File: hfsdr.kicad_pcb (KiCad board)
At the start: 2 copper layers, 91 parts, among them J1 RFIN, U2 ADA4938-1, U4 AD9515

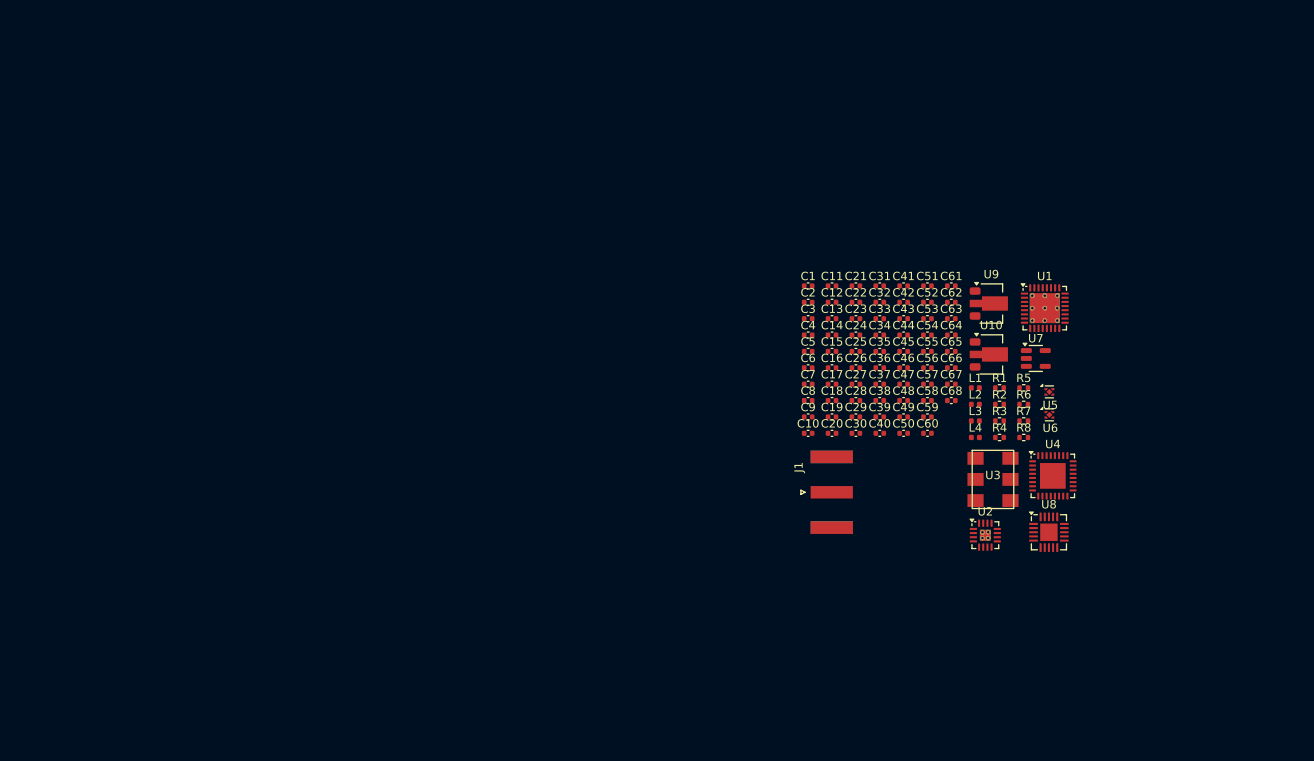
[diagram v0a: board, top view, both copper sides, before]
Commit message: dgfsd
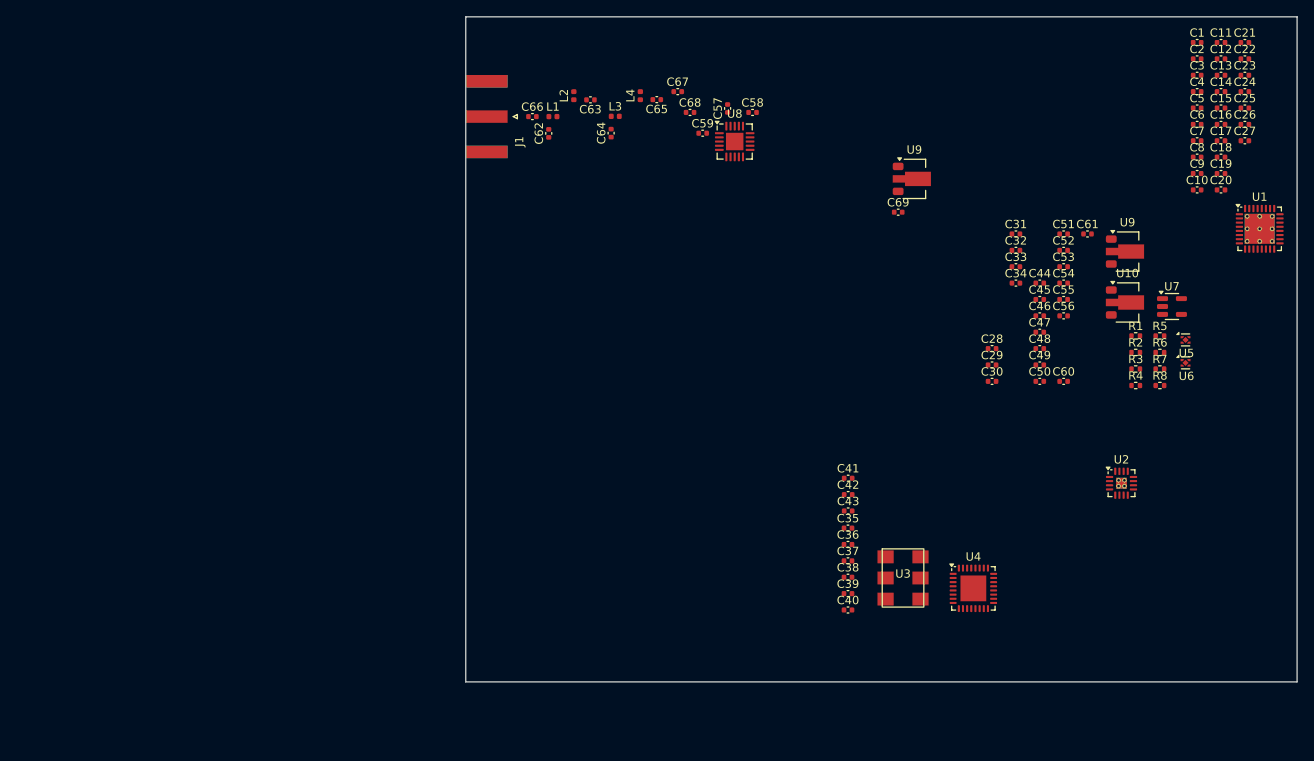
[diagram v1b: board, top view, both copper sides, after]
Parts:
- added C69: 0.1uF, Capacitor_SMD:C_0402_1005Metric, F.Cu at (167.0, 93.5)
- added U9: AP2205-50Y-13, Package_TO_SOT_SMD:SOT-89-3, F.Cu at (169.0, 89.5)
- U10: value ~ -> AP2205-50Y-13
- U7: value ~ -> TLV77333PDBVR
- U8: value ~ -> ADL5206
- moved J1 61.4 mm to (117.5, 82.0), turned to 180 degrees
- moved L2 60.9 mm to (128.0, 79.5), turned to 90 degrees
- moved L1 60.4 mm to (125.5, 82.0)
- moved U8 60.3 mm to (147.3, 85.0)
- moved C66 58.8 mm to (123.0, 82.0)
- moved L4 57.6 mm to (136.0, 79.5), turned to 90 degrees
- moved L3 56.7 mm to (133.0, 82.0)
- moved C1 55.2 mm to (203.0, 73.1)
- moved C10 55.2 mm to (203.0, 90.8)
- moved C11 55.2 mm to (205.8, 73.1)
- moved C12 55.2 mm to (205.8, 75.1)
- moved C13 55.2 mm to (205.8, 77.0)
- moved C14 55.2 mm to (205.8, 79.0)
- moved C15 55.2 mm to (205.8, 81.0)
- moved C16 55.2 mm to (205.8, 82.9)
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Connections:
- C19 pad 2: AGND -> DRGND
- C20 pad 2: AGND -> DRGND
- C21 pad 2: AGND -> DRGND
- C22 pad 2: AGND -> DRGND
- C23 pad 2: AGND -> DRGND
- C24 pad 2: AGND -> DRGND
- C25 pad 2: AGND -> DRGND
- C26 pad 2: AGND -> DRGND
- U2 pad 14: -5V -> -5V_1
- U2 pad 15: -5V -> -5V_3
- U2 pad 16: -5V -> -5V_2
- U8 pad 6: VGA_CSB -> unconnected-(U8-CS/GS1/D3-Pad6)
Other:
- board outline added: 100 x 80 mm
- copper layers 2 -> 4

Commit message: some more fpga work
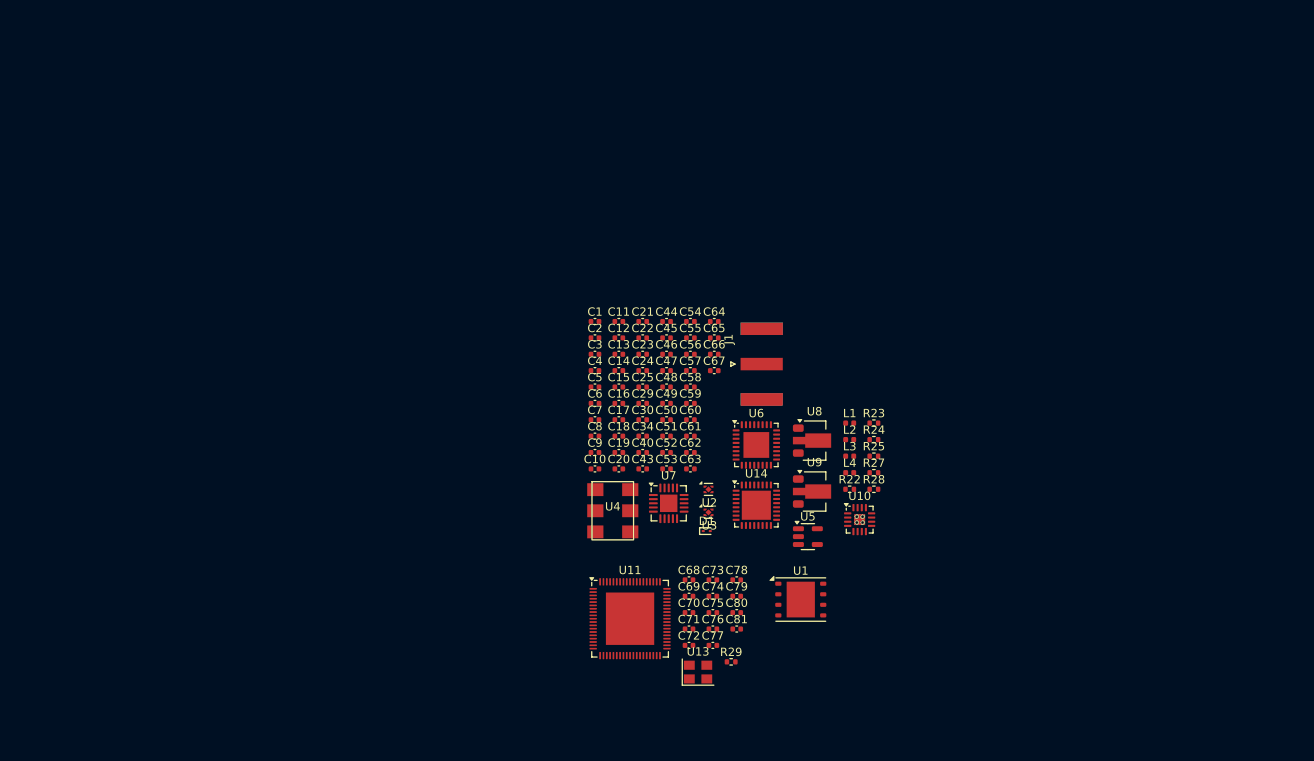
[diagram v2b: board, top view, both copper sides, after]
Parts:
- removed C26: 1uF, Capacitor_SMD:C_0402_1005Metric
- removed C27, C33, C35, C36, C37, C38, C39, C41, C42: 0.1uF, Capacitor_SMD:C_0402_1005Metric
- removed C28: 15pF, Capacitor_SMD:C_0402_1005Metric
- removed C31, C32: 0.1u, Capacitor_SMD:C_0402_1005Metric
- removed R1, R2: 250, Resistor_SMD:R_0402_1005Metric
- removed R3, R5: 33, Resistor_SMD:R_0402_1005Metric
- removed R4, R6: 15, Resistor_SMD:R_0402_1005Metric
- removed R7, R8: 50, Resistor_SMD:R_0402_1005Metric
- removed the U9 at (194.6, 98.2)
- removed the U9 at (169.0, 89.5)
- added C70: 100n, Capacitor_SMD:C_0402_1005Metric, F.Cu at (141.9, 141.7)
- added C71: 100n, Capacitor_SMD:C_0402_1005Metric, F.Cu at (141.9, 143.6)
- added C72: 100n, Capacitor_SMD:C_0402_1005Metric, F.Cu at (141.9, 145.6)
- added C73: 100u, Capacitor_SMD:C_0402_1005Metric, F.Cu at (144.7, 137.7)
- added C74: 4.7u, Capacitor_SMD:C_0402_1005Metric, F.Cu at (144.7, 139.7)
- added C75: 0.1u, Capacitor_SMD:C_0402_1005Metric, F.Cu at (144.7, 141.7)
- added C76: 0.1u, Capacitor_SMD:C_0402_1005Metric, F.Cu at (144.7, 143.6)
- added C77: 26p, Capacitor_SMD:C_0402_1005Metric, F.Cu at (144.7, 145.6)
- added C78: 26p, Capacitor_SMD:C_0402_1005Metric, F.Cu at (147.6, 137.7)
- added C79: 0.1uF, Capacitor_SMD:C_0402_1005Metric, F.Cu at (147.6, 139.7)
- added C80: 0.1uF, Capacitor_SMD:C_0402_1005Metric, F.Cu at (147.6, 141.7)
- added C81: 0.1uF, Capacitor_SMD:C_0402_1005Metric, F.Cu at (147.6, 143.6)
- added D1: ESD9B3.3ST5G, Diode_SMD:D_SOD-923, F.Cu at (144.0, 131.9)
- added R22: 50, Resistor_SMD:R_0402_1005Metric, F.Cu at (161.2, 126.8)
- added R23: 50, Resistor_SMD:R_0402_1005Metric, F.Cu at (164.1, 118.9)
- added R24: 250, Resistor_SMD:R_0402_1005Metric, F.Cu at (164.1, 120.9)
- added R25: 250, Resistor_SMD:R_0402_1005Metric, F.Cu at (164.1, 122.8)
- added R27: 33, Resistor_SMD:R_0402_1005Metric, F.Cu at (164.1, 124.8)
- added R28: 33, Resistor_SMD:R_0402_1005Metric, F.Cu at (164.1, 126.8)
- added R29: 1.6K 1%, Resistor_SMD:R_0402_1005Metric, F.Cu at (146.9, 147.6)
- added U11: FT601Q, Package_DFN_QFN:QFN-76-1EP_9x9mm_P0.4mm_EP5.81x6.31mm, F.Cu at (134.8, 142.4)
- added U13: ABM8-30.000MHZ-D1X-T, Oscillator:Oscillator_SMD_Abracon_ASE-4Pin_3.2x2.5mm, F.Cu at (142.9, 148.8)
- added U14: AD9649, Package_CSP:LFCSP-32-1EP_5x5mm_P0.5mm_EP3.5x3.5mm, F.Cu at (150.0, 128.8)
- added U9: AP2205-50Y-13, Package_TO_SOT_SMD:SOT-89-3, F.Cu at (157.0, 127.1)
- C10, C13, C15, C16, C17, C18, C24, C25, C34, C44, C45, C46, C49: value 1uF -> 0.1uF
- C19, C2, C5, C59, C6, C8, C9: value 0.1uF -> 1uF
- C29: value 5pF -> 1uF
- C30: value 15pF -> 0.1uF
- C47: value 1uF -> 0.1u
- C48: value 0.1uF -> 0.1u
- C51: value 0.1n -> 1uF
- C53: value 0.1uF -> 0.1n
- C57: value 0.1uF -> 470n
- C58: value 0.1uF -> 120p
- C60: value 1uF -> 200p
- C61: value 2.2uF -> 200p
- C62: value 120p -> 2.2uF
- C63: value 200p -> 160p
- C64: value 200p -> 0.1u
- C65: value 160p -> 0.1u
- C66: value 470n -> 0.1uF
- C67: value 0.1u -> 22pF
- C68: value 0.1u -> 100n
- C69: value 0.1uF -> 100n
- U1: value ~ -> W25Q128JVP; footprint Package_CSP:LFCSP-32-1EP_5x5mm_P0.5mm_EP3.6x3.6mm_ThermalVias -> Package_SON:WSON-8-1EP_6x5mm_P1.27mm_EP3.4x4.3mm
- U10: value AP2205-50Y-13 -> ADA4938-1; footprint Package_TO_SOT_SMD:SOT-89-3 -> Package_CSP:LFCSP-16-1EP_3x3mm_P0.5mm_EP1.3x1.3mm_ThermalVias
- U2: value ADA4938-1 -> ~; footprint Package_CSP:LFCSP-16-1EP_3x3mm_P0.5mm_EP1.3x1.3mm_ThermalVias -> Package_DFN_QFN:OnSemi_XDFN4-1EP_1.0x1.0mm_EP0.52x0.52mm
- U3: footprint hfsdr:SI590_5x7mm -> Package_DFN_QFN:OnSemi_XDFN4-1EP_1.0x1.0mm_EP0.52x0.52mm
- U4: value AD9515 -> ~; footprint Package_CSP:LFCSP-32-1EP_5x5mm_P0.5mm_EP3.1x3.1mm -> hfsdr:SI590_5x7mm
- U5: value ~ -> TLV77333PDBVR; footprint Package_DFN_QFN:OnSemi_XDFN4-1EP_1.0x1.0mm_EP0.52x0.52mm -> Package_TO_SOT_SMD:SOT-23-5
- U6: value ~ -> AD9515; footprint Package_DFN_QFN:OnSemi_XDFN4-1EP_1.0x1.0mm_EP0.52x0.52mm -> Package_CSP:LFCSP-32-1EP_5x5mm_P0.5mm_EP3.1x3.1mm
- U7: value TLV77333PDBVR -> ADL5206; footprint Package_TO_SOT_SMD:SOT-23-5 -> Package_CSP:LFCSP-20-1EP_4x4mm_P0.5mm_EP2.1x2.1mm
- U8: value ADL5206 -> AP2205-50Y-13; footprint Package_CSP:LFCSP-20-1EP_4x4mm_P0.5mm_EP2.1x2.1mm -> Package_TO_SOT_SMD:SOT-89-3
- moved C1 79.8 mm to (130.5, 106.7)
- moved C10 79.8 mm to (130.5, 124.4)
- moved C11 79.8 mm to (133.4, 106.7)
- moved C12 79.8 mm to (133.4, 108.6)
- moved C13 79.8 mm to (133.4, 110.6)
- moved C14 79.8 mm to (133.4, 112.6)
- moved C15 79.8 mm to (133.4, 114.5)
- moved C16 79.8 mm to (133.4, 116.5)
- moved C17 79.8 mm to (133.4, 118.5)
- moved C18 79.8 mm to (133.4, 120.4)
- moved C19 79.8 mm to (133.4, 122.4)
- moved C2 79.8 mm to (130.5, 108.6)
- moved C20 79.8 mm to (133.4, 124.4)
- moved C21 79.8 mm to (136.3, 106.7)
- moved C22 79.8 mm to (136.3, 108.6)
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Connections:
- C10 pad 1: AVDD -> CLKVDD
- C12 pad 1: AVDD -> DRVDD
- C15 pad 1: AVDD -> VCM
- C16 pad 1: AVDD -> CLKVDD
- C18 pad 1: AVDD -> VREF
- C19 pad 1: DRVDD -> VREF
- C19 pad 2: DRGND -> AGND
- C20 pad 1: DRVDD -> CLKVDD
- C20 pad 2: DRGND -> AGND
- C21 pad 1: DRVDD -> Net-(C21-Pad1)
- C21 pad 2: DRGND -> CLK-
- C22 pad 1: DRVDD -> Net-(C22-Pad1)
- C22 pad 2: DRGND -> CLK+
- C23 pad 2: DRGND -> AGND
- C24 pad 1: DRVDD -> CLKVDD
- C24 pad 2: DRGND -> AGND
- C25 pad 1: DRVDD -> CLKVDD
- C25 pad 2: DRGND -> AGND
- C29 pad 1: Net-(C29-Pad1) -> CLKVDD
- C29 pad 2: Net-(C28-Pad1) -> AGND
- C3 pad 1: AVDD -> DRVDD
- C30 pad 1: AGND -> CLKVDD
- C30 pad 2: Net-(C29-Pad1) -> AGND
- C4 pad 1: AVDD -> CLKVDD
- C44 pad 1: +5V -> VCM
- C45 pad 1: AVDD -> VGA_VDD
- C46 pad 1: +5V -> AGND
- C46 pad 2: AGND -> Net-(U6-S6)
- C47 pad 1: DRVDD -> Net-(U4-CLK+)
- C47 pad 2: AGND -> Net-(U6-CLK)
- C48 pad 1: AGND -> Net-(U4-CLK-)
- C48 pad 2: Net-(U4-S6) -> Net-(U6-CLKB)
- C49 pad 1: +5V -> VGA_VDD
- C5 pad 1: AVDD -> +5V
- C50 pad 1: CLKVDD -> +5V
- C51 pad 1: Net-(U4-OUT0B) -> CLKVDD
- C51 pad 2: CLK- -> AGND
- C52 pad 1: Net-(U4-OUT0) -> Net-(U6-OUT0B)
- C52 pad 2: CLK+ -> Net-(C21-Pad1)
- C53 pad 1: Net-(U1-CLK-) -> Net-(U6-OUT0)
- C53 pad 2: CLK- -> Net-(C22-Pad1)
- C54 pad 1: Net-(U1-CLK+) -> AGND
- C54 pad 2: CLK+ -> Net-(U7-VCM)
- C57 pad 1: VGA_VDD -> Net-(D1-A2)
- C57 pad 2: AGND -> Net-(C57-Pad2)
- C58 pad 1: VGA_VDD -> Net-(C57-Pad2)
- C59 pad 1: AGND -> +13.8V
- C59 pad 2: Net-(U8-VCM) -> AGND
- C6 pad 1: AVDD -> +5V
- C60 pad 1: +13.8V -> Net-(C60-Pad1)
- C61 pad 1: Net-(U10-VOUT) -> Net-(C61-Pad1)
- C62 pad 1: Net-(C62-Pad1) -> Net-(U9-VOUT)
- C64 pad 2: AGND -> AMPIN+
- C65 pad 1: Net-(C65-Pad1) -> AGND
- C65 pad 2: AGND -> AMPIN-
- C66 pad 1: Net-(J1-In) -> AGND
- C66 pad 2: Net-(C62-Pad1) -> Net-(U9-VOUT)
- C67 pad 1: Net-(C67-Pad1) -> ADCIN-
- C67 pad 2: AMPIN+ -> ADCIN+
- C68 pad 1: AGND -> Net-(J2-TX1-)
- C68 pad 2: AMPIN- -> Net-(U12-TX1n)
- C69 pad 1: AGND -> Net-(J2-TX1+)
- C69 pad 2: Net-(U10-VOUT) -> Net-(U12-TX1p)
- J1 pad 1: Net-(J1-In) -> Net-(D1-A2)
- L1 pad 1: Net-(C62-Pad1) -> Net-(C57-Pad2)
- L1 pad 2: Net-(C63-Pad1) -> Net-(C60-Pad1)
- L2 pad 1: Net-(C63-Pad1) -> Net-(C60-Pad1)
- L2 pad 2: Net-(C64-Pad1) -> Net-(C61-Pad1)
- L3 pad 1: Net-(C64-Pad1) -> Net-(C61-Pad1)
- L3 pad 2: Net-(C65-Pad1) -> Net-(C63-Pad1)
- L4 pad 1: Net-(C65-Pad1) -> Net-(C63-Pad1)
- L4 pad 2: Net-(C67-Pad1) -> Net-(C64-Pad1)
- U1 pad 1: AVDD -> unconnected-(U1-~{CS}-Pad1)
- U1 pad 3: AVDD -> unconnected-(U1-IO2-Pad3)
- U1 pad 4: Net-(U1-CLK+) -> unconnected-(U1-GND-Pad4)
- U1 pad 5: Net-(U1-CLK-) -> unconnected-(U1-DI(IO0)-Pad5)
- U1 pad 6: AVDD -> unconnected-(U1-CLK-Pad6)
- U1 pad 8: AVDD -> unconnected-(U1-VCC-Pad8)
- U1 pad 9: unconnected-(U1-DSYNC--Pad9) -> (no net)
- U10 pad 1: +13.8V -> Net-(U10A-FB-)
- U10 pad 2: AGND -> Net-(U10A-+)
- U10 pad 3: Net-(U10-VOUT) -> Net-(U10A--)
- U2 pad 1: Net-(U2A-FB-) -> AVDD
- U2 pad 2: Net-(U2A-+) -> AGND
- U2 pad 4: Net-(U2A-FB+) -> +5V
- U2 pad 5: Net-(U10-VOUT) -> AGND
- U3 pad 1: unconnected-(U3-NC-Pad1) -> DRVDD
- U3 pad 2: Net-(U3-OE) -> AGND
- U3 pad 3: AGND -> Net-(U3-EN)
- U3 pad 4: Net-(U3-CLK+) -> +5V
- U3 pad 5: Net-(U3-CLK-) -> AGND
- U4 pad 1: CLKVDD -> unconnected-(U4-NC-Pad1)
- U4 pad 3: Net-(U4-CLKB) -> AGND
- U4 pad 4: CLKVDD -> Net-(U4-CLK+)
- U4 pad 5: Net-(U4-SYNCB) -> Net-(U4-CLK-)
- U4 pad 6: unconnected-(U4-VREF-Pad6) -> CLKVDD
- U5 pad 1: AVDD -> +5V
- U5 pad 4: +5V -> unconnected-(U5-NC-Pad4)
- U5 pad 5: AGND -> CLKVDD
- U6 pad 1: DRVDD -> CLKVDD
- U6 pad 2: AGND -> Net-(U6-CLK)
- U6 pad 3: Net-(U6-EN) -> Net-(U6-CLKB)
- U6 pad 4: +5V -> CLKVDD
- U6 pad 5: AGND -> Net-(U6-SYNCB)
- U7 pad 1: +5V -> Net-(U7-VCM)
- U7 pad 2: AGND -> Net-(U7-MODE1)
- U7 pad 5: CLKVDD -> unconnected-(U7-SCLK/D4-Pad5)
- U8 pad 1: Net-(U8-VCM) -> +13.8V
- U8 pad 2: Net-(U8-MODE1) -> AGND
- U8 pad 3: Net-(U8-MODE0) -> VGA_VDD
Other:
- board outline removed

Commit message: i dont even remember what i did
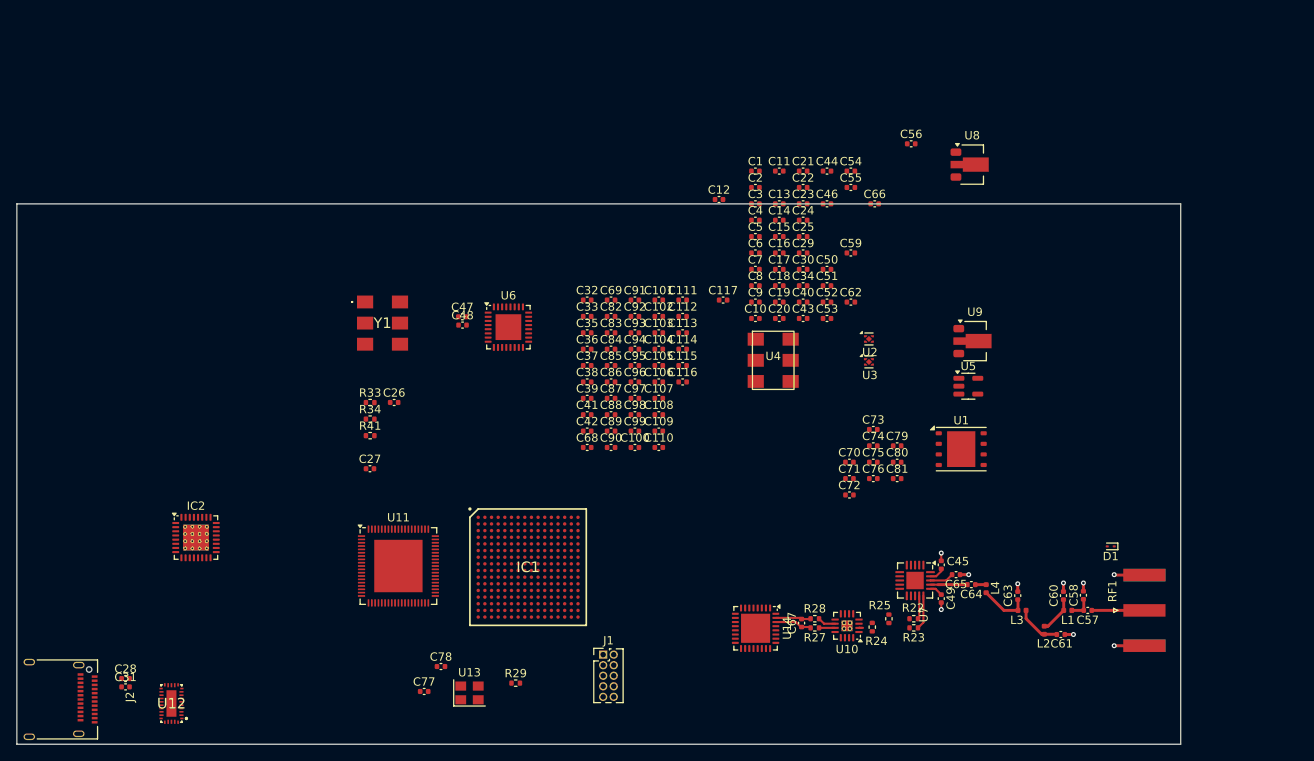
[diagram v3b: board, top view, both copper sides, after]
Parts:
- added C100: 0.1u, Capacitor_SMD:C_0402_1005Metric, F.Cu at (135.3, 121.8)
- added C101: 10u, Capacitor_SMD:C_0402_1005Metric, F.Cu at (138.2, 104.1)
- added C102: 0.1u, Capacitor_SMD:C_0402_1005Metric, F.Cu at (138.2, 106.0)
- added C103: 10u, Capacitor_SMD:C_0402_1005Metric, F.Cu at (138.2, 108.0)
- added C104: 0.1u, Capacitor_SMD:C_0402_1005Metric, F.Cu at (138.2, 110.0)
- added C105: 10u, Capacitor_SMD:C_0402_1005Metric, F.Cu at (138.2, 112.0)
- added C106: 0.1u, Capacitor_SMD:C_0402_1005Metric, F.Cu at (138.2, 113.9)
- added C107: 10u, Capacitor_SMD:C_0402_1005Metric, F.Cu at (138.2, 115.9)
- added C108: 0.1u, Capacitor_SMD:C_0402_1005Metric, F.Cu at (138.2, 117.9)
- added C109: 10u, Capacitor_SMD:C_0402_1005Metric, F.Cu at (138.2, 119.8)
- added C110: 0.1u, Capacitor_SMD:C_0402_1005Metric, F.Cu at (138.2, 121.8)
- added C111: 10u, Capacitor_SMD:C_0402_1005Metric, F.Cu at (141.1, 104.1)
- added C112: 0.1u, Capacitor_SMD:C_0402_1005Metric, F.Cu at (141.1, 106.0)
- added C113: 10u, Capacitor_SMD:C_0402_1005Metric, F.Cu at (141.1, 108.0)
- added C114: 0.1u, Capacitor_SMD:C_0402_1005Metric, F.Cu at (141.1, 110.0)
- added C115: 10u, Capacitor_SMD:C_0402_1005Metric, F.Cu at (141.1, 112.0)
- added C116: 0.1u, Capacitor_SMD:C_0402_1005Metric, F.Cu at (141.1, 113.9)
- added C117: 1000p, Capacitor_SMD:C_0402_1005Metric, F.Cu at (146.0, 104.1)
- added C26: 100n, Capacitor_SMD:C_0402_1005Metric, F.Cu at (106.4, 116.4)
- added C27: 0.1u, Capacitor_SMD:C_0402_1005Metric, F.Cu at (103.5, 124.4)
- added C28: 100n, Capacitor_SMD:C_0402_1005Metric, F.Cu at (74.1, 149.6)
- added C31: 100n, Capacitor_SMD:C_0402_1005Metric, F.Cu at (74.1, 150.6)
- added C32: 10u, Capacitor_SMD:C_0402_1005Metric, F.Cu at (129.6, 104.1)
- added C33: 10u, Capacitor_SMD:C_0402_1005Metric, F.Cu at (129.6, 106.0)
- added C35: 10u, Capacitor_SMD:C_0402_1005Metric, F.Cu at (129.6, 108.0)
- added C36: 0.1u, Capacitor_SMD:C_0402_1005Metric, F.Cu at (129.6, 110.0)
- added C37: 10u, Capacitor_SMD:C_0402_1005Metric, F.Cu at (129.6, 112.0)
- added C38: 10u, Capacitor_SMD:C_0402_1005Metric, F.Cu at (129.6, 113.9)
- added C39: 10u, Capacitor_SMD:C_0402_1005Metric, F.Cu at (129.6, 115.9)
- added C41: 0.1u, Capacitor_SMD:C_0402_1005Metric, F.Cu at (129.6, 117.9)
- added C42: 10u, Capacitor_SMD:C_0402_1005Metric, F.Cu at (129.6, 119.8)
- added C82: 0.1u, Capacitor_SMD:C_0402_1005Metric, F.Cu at (132.5, 106.0)
- added C83: 10u, Capacitor_SMD:C_0402_1005Metric, F.Cu at (132.5, 108.0)
- added C84: 10u, Capacitor_SMD:C_0402_1005Metric, F.Cu at (132.5, 110.0)
- added C85: 10u, Capacitor_SMD:C_0402_1005Metric, F.Cu at (132.5, 112.0)
- added C86: 10u, Capacitor_SMD:C_0402_1005Metric, F.Cu at (132.5, 113.9)
- added C87: 10u, Capacitor_SMD:C_0402_1005Metric, F.Cu at (132.5, 115.9)
- added C88: 10u, Capacitor_SMD:C_0402_1005Metric, F.Cu at (132.5, 117.9)
- added C89: 10u, Capacitor_SMD:C_0402_1005Metric, F.Cu at (132.5, 119.8)
- added C90: 10u, Capacitor_SMD:C_0402_1005Metric, F.Cu at (132.5, 121.8)
- added C91: 10u, Capacitor_SMD:C_0402_1005Metric, F.Cu at (135.3, 104.1)
- added C92: 0.1u, Capacitor_SMD:C_0402_1005Metric, F.Cu at (135.3, 106.0)
- added C93: 0.1u, Capacitor_SMD:C_0402_1005Metric, F.Cu at (135.3, 108.0)
- added C94: 0.1u, Capacitor_SMD:C_0402_1005Metric, F.Cu at (135.3, 110.0)
- added C95: 10u, Capacitor_SMD:C_0402_1005Metric, F.Cu at (135.3, 112.0)
- added C96: 0.1u, Capacitor_SMD:C_0402_1005Metric, F.Cu at (135.3, 113.9)
- added C97: 10u, Capacitor_SMD:C_0402_1005Metric, F.Cu at (135.3, 115.9)
- added C98: 0.1u, Capacitor_SMD:C_0402_1005Metric, F.Cu at (135.3, 117.9)
- added C99: 10u, Capacitor_SMD:C_0402_1005Metric, F.Cu at (135.3, 119.8)
- added IC1: LFE5U-25F-6BG256C, hfsdr:BGA256C80P16X16_1400X1400X170, F.Cu at (122.5, 136.2)
- added IC2: AD9707BCPZ, Package_CSP:LFCSP-32-1EP_5x5mm_P0.5mm_EP3.1x3.1mm_ThermalVias, F.Cu at (82.5, 132.6)
- added J1: JTAG, Connector_PinHeader_1.27mm:PinHeader_2x05_P1.27mm_Vertical, F.Cu at (131.5, 146.7)
- added J2: GSB4D313302Y1HR, Connector_USB:USB_C_Receptacle_Amphenol_12401610E4-2A, F.Cu at (65.3, 152.1)
- added R33: 10K, Resistor_SMD:R_0402_1005Metric, F.Cu at (103.5, 116.4)
- added R34: 10K, Resistor_SMD:R_0402_1005Metric, F.Cu at (103.5, 118.4)
- added R41: 10K, Resistor_SMD:R_0402_1005Metric, F.Cu at (103.5, 120.4)
- added U12: HD3SS3220, hfsdr:HD3SS3220IRNHR, F.Cu at (79.6, 152.6)
- added Y1: 590BD80M0000DG, hfsdr:590BD80M0000DG, F.Cu at (105.0, 106.8)
- C68, C69: value 100n -> 10u
- moved C57 55.8 mm to (189.8, 141.4), turned to 180 degrees
- moved RF1 54.7 mm to (196.6, 141.4)
- moved C58 53.5 mm to (189.3, 139.6), turned to 90 degrees
- moved C61 50.5 mm to (186.6, 144.3)
- moved C60 49.6 mm to (186.9, 139.6), turned to 90 degrees
- moved D1 48.6 mm to (192.6, 133.7), turned to 180 degrees
- moved C64 44.3 mm to (175.8, 138.3), turned to 180 degrees
- moved C45 42.9 mm to (172.2, 135.9), turned to 90 degrees
- moved C63 42.2 mm to (181.4, 139.6), turned to 90 degrees
- moved C65 40.7 mm to (174.0, 137.1), turned to 180 degrees
- moved C49 40.5 mm to (172.2, 140.0), turned to -90 degrees
- moved U8 38.2 mm to (175.9, 87.8)
- moved C78 37.1 mm to (112.0, 148.2)
- moved C69 36.8 mm to (132.5, 104.1)
- moved C56 36.7 mm to (168.6, 85.3)
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- renumbered J1 to RF1
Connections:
- net OE_N renamed FT_OEn
- net RD_N renamed FT_RDn
- net RXF_N renamed FT_RXFn
- net TXE_N renamed FT_TXEn
- net WR_N renamed FT_WRn
- C47 pad 1: Net-(U4-CLK+) -> Net-(Y1-CLK+)
- C48 pad 1: Net-(U4-CLK-) -> Net-(Y1-CLK-)
- C68 pad 1: Net-(J2-TX1-) -> P1.1V
- C68 pad 2: Net-(U12-TX1n) -> AGND
- C69 pad 1: Net-(J2-TX1+) -> P1.1V
- C69 pad 2: Net-(U12-TX1p) -> AGND
- C70 pad 1: Net-(J2-TX2-) -> TX2-
- C71 pad 1: Net-(J2-TX2+) -> TX2+
- C72 pad 1: GND -> AGND
- C73 pad 2: GND -> AGND
- C74 pad 1: GND -> AGND
- C77 pad 1: GND -> AGND
- C78 pad 1: GND -> AGND
- C79 pad 1: GND -> AGND
- C80 pad 1: GND -> AGND
- C81 pad 1: GND -> AGND
- R22 pad 2: Net-(U10A--) -> Net-(U10A-+)
- R23 pad 2: Net-(U10A-+) -> Net-(U10A--)
- R24 pad 1: Net-(U10A--) -> Net-(U10A-+)
- R25 pad 1: Net-(U10A-+) -> Net-(U10A--)
- R29 pad 1: GND -> AGND
- U1 pad 1: unconnected-(U1-~{CS}-Pad1) -> SPICFG_SS
- U1 pad 2: unconnected-(U1-DO(IO1)-Pad2) -> SPICFG_MISO
- U1 pad 3: unconnected-(U1-IO2-Pad3) -> QSPI_D2
- U1 pad 4: unconnected-(U1-GND-Pad4) -> AGND
- U1 pad 5: unconnected-(U1-DI(IO0)-Pad5) -> SPICFG_MOSI
- U1 pad 6: unconnected-(U1-CLK-Pad6) -> SPICFG_SCK
- U1 pad 7: unconnected-(U1-IO3-Pad7) -> QSPI_D3
- U1 pad 8: unconnected-(U1-VCC-Pad8) -> P3.3V
- U10 pad 17: unconnected-(U10B-PAD-Pad17) -> -5V
- U11 pad 1: GND -> AGND
- U11 pad 10: Net-(U11-~{SIWU}) -> FT_SIWUn
- U11 pad 15: Net-(U11-~{RESET}) -> FT_RESETn
- U11 pad 16: USB_WAKEUP -> FT_WAKEUPn
- U11 pad 17: FT_GPIO0 -> unconnected-(U11-GPIO0-Pad17)
- U11 pad 18: FT_GPIO1 -> unconnected-(U11-GPIO1-Pad18)
- U11 pad 26: GND -> AGND
- U11 pad 29: GND -> AGND
- U11 pad 36: GND -> AGND
- U11 pad 4: unconnected-(U11-BE_0-Pad4) -> FT_BE0
- U11 pad 40: unconnected-(U11-DATA_0-Pad40) -> FT_D0
- U11 pad 41: unconnected-(U11-DATA_1-Pad41) -> FT_D1
- U11 pad 42: unconnected-(U11-DATA_2-Pad42) -> FT_D2
- U11 pad 43: unconnected-(U11-DATA_3-Pad43) -> FT_D3
- U11 pad 44: unconnected-(U11-DATA_4-Pad44) -> FT_D4
- U11 pad 45: unconnected-(U11-DATA_5-Pad45) -> FT_D5
- U11 pad 46: unconnected-(U11-DATA_6-Pad46) -> FT_D6
- U11 pad 47: unconnected-(U11-DATA_7-Pad47) -> FT_D7
- U11 pad 5: unconnected-(U11-BE_1-Pad5) -> FT_BE1
- U11 pad 50: unconnected-(U11-DATA_8-Pad50) -> FT_D8
- U11 pad 51: unconnected-(U11-DATA_9-Pad51) -> FT_D9
- U11 pad 52: unconnected-(U11-DATA_10-Pad52) -> FT_D10
- U11 pad 53: unconnected-(U11-DATA_11-Pad53) -> FT_D11
- U11 pad 54: unconnected-(U11-DATA_12-Pad54) -> FT_D12
- U11 pad 55: unconnected-(U11-DATA_13-Pad55) -> FT_D13
- U11 pad 56: unconnected-(U11-DATA_14-Pad56) -> FT_D14
- U11 pad 57: unconnected-(U11-DATA_15-Pad57) -> FT_D15
- U11 pad 58: unconnected-(U11-CLK-Pad58) -> Net-(U11-CLK)
- U11 pad 6: unconnected-(U11-BE_2-Pad6) -> FT_BE2
- U11 pad 60: unconnected-(U11-DATA_16-Pad60) -> FT_D16
- U11 pad 61: unconnected-(U11-DATA_17-Pad61) -> FT_D17
- U11 pad 62: unconnected-(U11-DATA_18-Pad62) -> FT_D18
- U11 pad 63: unconnected-(U11-DATA_19-Pad63) -> FT_D19
- U11 pad 64: unconnected-(U11-DATA_20-Pad64) -> FT_D20
- U11 pad 65: unconnected-(U11-DATA_21-Pad65) -> FT_D21
- U11 pad 66: unconnected-(U11-DATA_22-Pad66) -> FT_D22
- U11 pad 67: unconnected-(U11-DATA_23-Pad67) -> FT_D23
- U11 pad 69: unconnected-(U11-DATA_24-Pad69) -> FT_D24
- U11 pad 7: unconnected-(U11-BE_3-Pad7) -> FT_BE3
- U11 pad 70: unconnected-(U11-DATA_25-Pad70) -> FT_D25
- U11 pad 71: unconnected-(U11-DATA_26-Pad71) -> FT_D26
- U11 pad 72: unconnected-(U11-DATA_27-Pad72) -> FT_D27
- U11 pad 73: unconnected-(U11-DATA_28-Pad73) -> FT_D28
- U11 pad 74: unconnected-(U11-DATA_29-Pad74) -> FT_D29
- U11 pad 75: unconnected-(U11-DATA_30-Pad75) -> FT_D30
- U11 pad 76: unconnected-(U11-DATA_31-Pad76) -> FT_D31
- U11 pad 77: GND -> AGND
- U13 pad 2: GND -> AGND
- U13 pad 4: GND -> AGND
- U14 pad 23: unconnected-(U14-MODE/OR-Pad23) -> ADC_MODE/OR
- U14 pad 33: (no net) -> AGND
- U14 pad 5: unconnected-(U14-SCLK/DFS-Pad5) -> ADC_SCLK
- U14 pad 6: unconnected-(U14-SDIO/PDWN-Pad6) -> ADC_SDIO
- U7 pad 4: unconnected-(U7-SDIO/SDO-Pad4) -> VGA_SDIO
- U7 pad 5: unconnected-(U7-SCLK/D4-Pad5) -> VGA_SCLK
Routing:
- net AGND: track 0.00 -> 13.9 mm, vias 0 -> 9
- net Net-(D1-A2): track 0.00 -> 6.34 mm
- net Net-(C63-Pad1): track 0.00 -> 6.02 mm
- net Net-(C61-Pad1): track 0.00 -> 5.48 mm
- net Net-(C60-Pad1): track 0.00 -> 4.47 mm
- net ADCIN-: track 0.00 -> 4.47 mm
- net AMPIN+: track 0.00 -> 4.44 mm
- net ADCIN+: track 0.00 -> 4.25 mm
- net Net-(U7-VOUT+): track 0.00 -> 4.12 mm
- net VGA_VDD: track 0.00 -> 3.43 mm
- net AMPIN-: track 0.00 -> 2.89 mm
- net Net-(C57-Pad2): track 0.00 -> 2.85 mm
- net Net-(U7-VOUT-): track 0.00 -> 2.81 mm
- net Net-(R28-Pad1): track 0.00 -> 2.17 mm
- net Net-(R27-Pad1): track 0.00 -> 1.93 mm
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- added copper zone on In1.Cu, net AGND
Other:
- board outline added: 140 x 65 mm
